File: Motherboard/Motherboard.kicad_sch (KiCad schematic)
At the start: 0 parts

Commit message: does like everything
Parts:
- added C1, C3, C4: 10uF, PCM_JLCPCB:C_0805, symbol PCM_JLCPCB-Capacitors:0805,10uF
- added C2, C5, C6, C8: 100nF, PCM_JLCPCB:C_0805, symbol PCM_JLCPCB-Capacitors:0805,100nF
- added C7: 1uF, PCM_JLCPCB:C_0805, symbol PCM_JLCPCB-Capacitors:0805,1uF
- added D1: 1N5819WS, PCM_JLCPCB:D_SOD-323, symbol PCM_JLCPCB-Diodes:Schottky,1N5819WS
- added D2: Yellow, PCM_JLCPCB:D_0805, symbol PCM_JLCPCB-Diodes:LED,0805,Yellow
- added J1: GSB316441CEU, GSB316441CEU:AMPHENOL_GSB316441CEU, symbol GSB316441CEU:GSB316441CEU
- added J2, J3, J4, J5: B3B-XH-A_LF__SN_, B3B-XH-A_LF__SN_:JST_B3B-XH-A_LF__SN_, symbol B3B-XH-A_LF__SN_:B3B-XH-A_LF__SN_
- added LS1: CMT-7525-80-SMT-TR, CMT-7525-80-SMT-TR_CUD, symbol CMT-7525-80-SMT:CMT-7525-80-SMT-TR
- added Q1: HL3400A, PCM_JLCPCB:Q_SOT-23, symbol PCM_JLCPCB-Transistors:NMOS,HL3400A
- added R1: 270Ω, PCM_JLCPCB:R_0805, symbol PCM_JLCPCB-Resistors:0805,270Ω
- added R2, R3: 10kΩ, PCM_JLCPCB:R_0805, symbol PCM_JLCPCB-Resistors:0805,10kΩ
- added R4: 100Ω, PCM_JLCPCB:R_0805, symbol PCM_JLCPCB-Resistors:0805,100Ω
- added R5: 100kΩ, PCM_JLCPCB:R_0805, symbol PCM_JLCPCB-Resistors:0805,100kΩ
- added S1, S2: Tactile Button, 160gf, PCM_JLCPCB:SW-SMD_4P-L5.1-W5.1-P3.70-LS6.5-TL-2, symbol PCM_JLCPCB-Connectors_Buttons:Tactile Button, 160gf
- added U1: ESP32-S3-WROOM-1, RF_Module:ESP32-S3-WROOM-1, symbol RF_Module:ESP32-S3-WROOM-1
- added U2: USBLC6-2P6, Package_TO_SOT_SMD:SOT-666, symbol Power_Protection:USBLC6-2P6
- added U3: AMS1117, PCM_JLCPCB:SOT-223-3_L6.5-W3.4-P2.30-LS7.0-BR, symbol PCM_JLCPCB-Power:LDO, 3.3V, 1A
- added U4: MCP73831-2-MC, Package_DFN_QFN:DFN-8-1EP_3x2mm_P0.5mm_EP1.7x1.4mm, symbol Battery_Management:MCP73831-2-MC
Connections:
- new net: Q1.1 (G), R4.1
- new net: LS1.1, Q1.3 (D)
- new net: D1.2, J1.1 (VBUS), U2.5 (VBUS)
- new net: J1.2 (D-), U2.6 (I/O1)
- new net: J1.3 (D+), U2.4 (I/O2)
- new net: C2.1, C3.1, C4.1, C5.1, LS1.2, R1.1, R2.1, R3.1, U1.2 (3V3), U3.2 (VOUT), U3.4 (VOUT)
- new net: R2.2, S1.1 (A), S1.2 (B), U1.27 (IO0)
- new net: D2.2, R1.2
- new net: U1.13 (USB_D-), U2.1 (I/O1)
- new net: U1.14 (USB_D+), U2.3 (I/O2)
- new net: R4.2, R5.1, U1.20 (IO12)
- new net: J2.1, U1.21 (IO13)
- new net: J3.1, U1.22 (IO14)
- new net: C7.1, R3.2, S2.1 (A), S2.2 (B), U1.3 (EN)
- new net: J4.1, U1.8 (IO15)
- new net: J5.1, U1.9 (IO16)
- new net: C1.1, D1.1, J2.2, J3.2, J4.2, J5.2, U3.3 (VIN), U4.1 (V_{DD}), U4.2 (V_{DD})
- new net: U4.3 (V_{BAT}), U4.4 (V_{BAT})
- new net: C6.1, S1.3 (C), S1.4 (D)
- new net: C8.1, S2.3 (C), S2.4 (D)
- new net GND: C1.2, C2.2, C3.2, C4.2, C5.2, C6.2, C7.2, C8.2, D2.1, J1.4 (GND), J1.7 (GND_DRAIN), J1.SH1 (SHIELD), J1.SH2 (SHIELD__1), J2.3, J3.3, J4.3, J5.3, Q1.2 (S), R5.2, U1.1 (GND), U1.40 (GND), U1.41 (GND), U2.2 (GND), U3.1 (GND), U4.6 (V_{SS})
- no-connect marks 0 -> 34

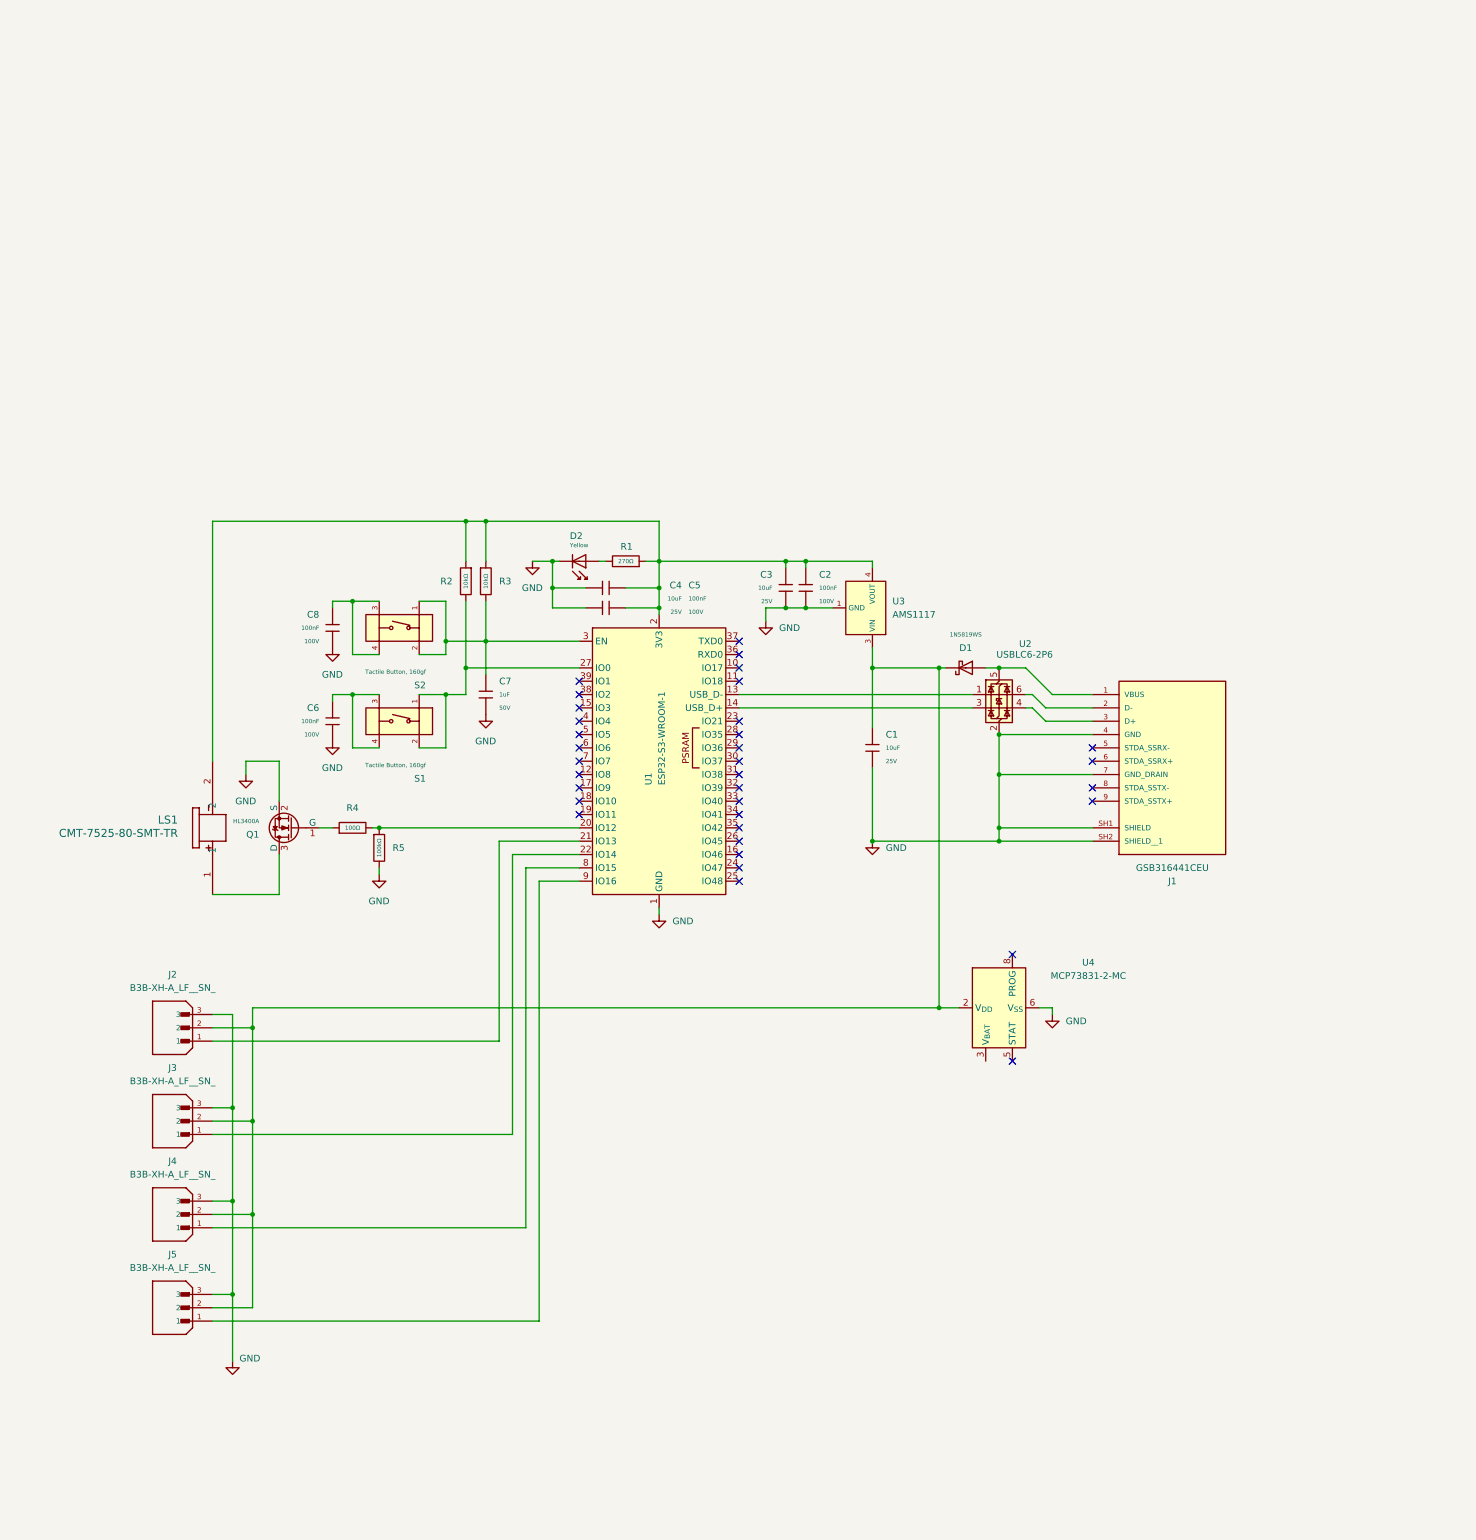
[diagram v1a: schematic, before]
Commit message: adds bms system
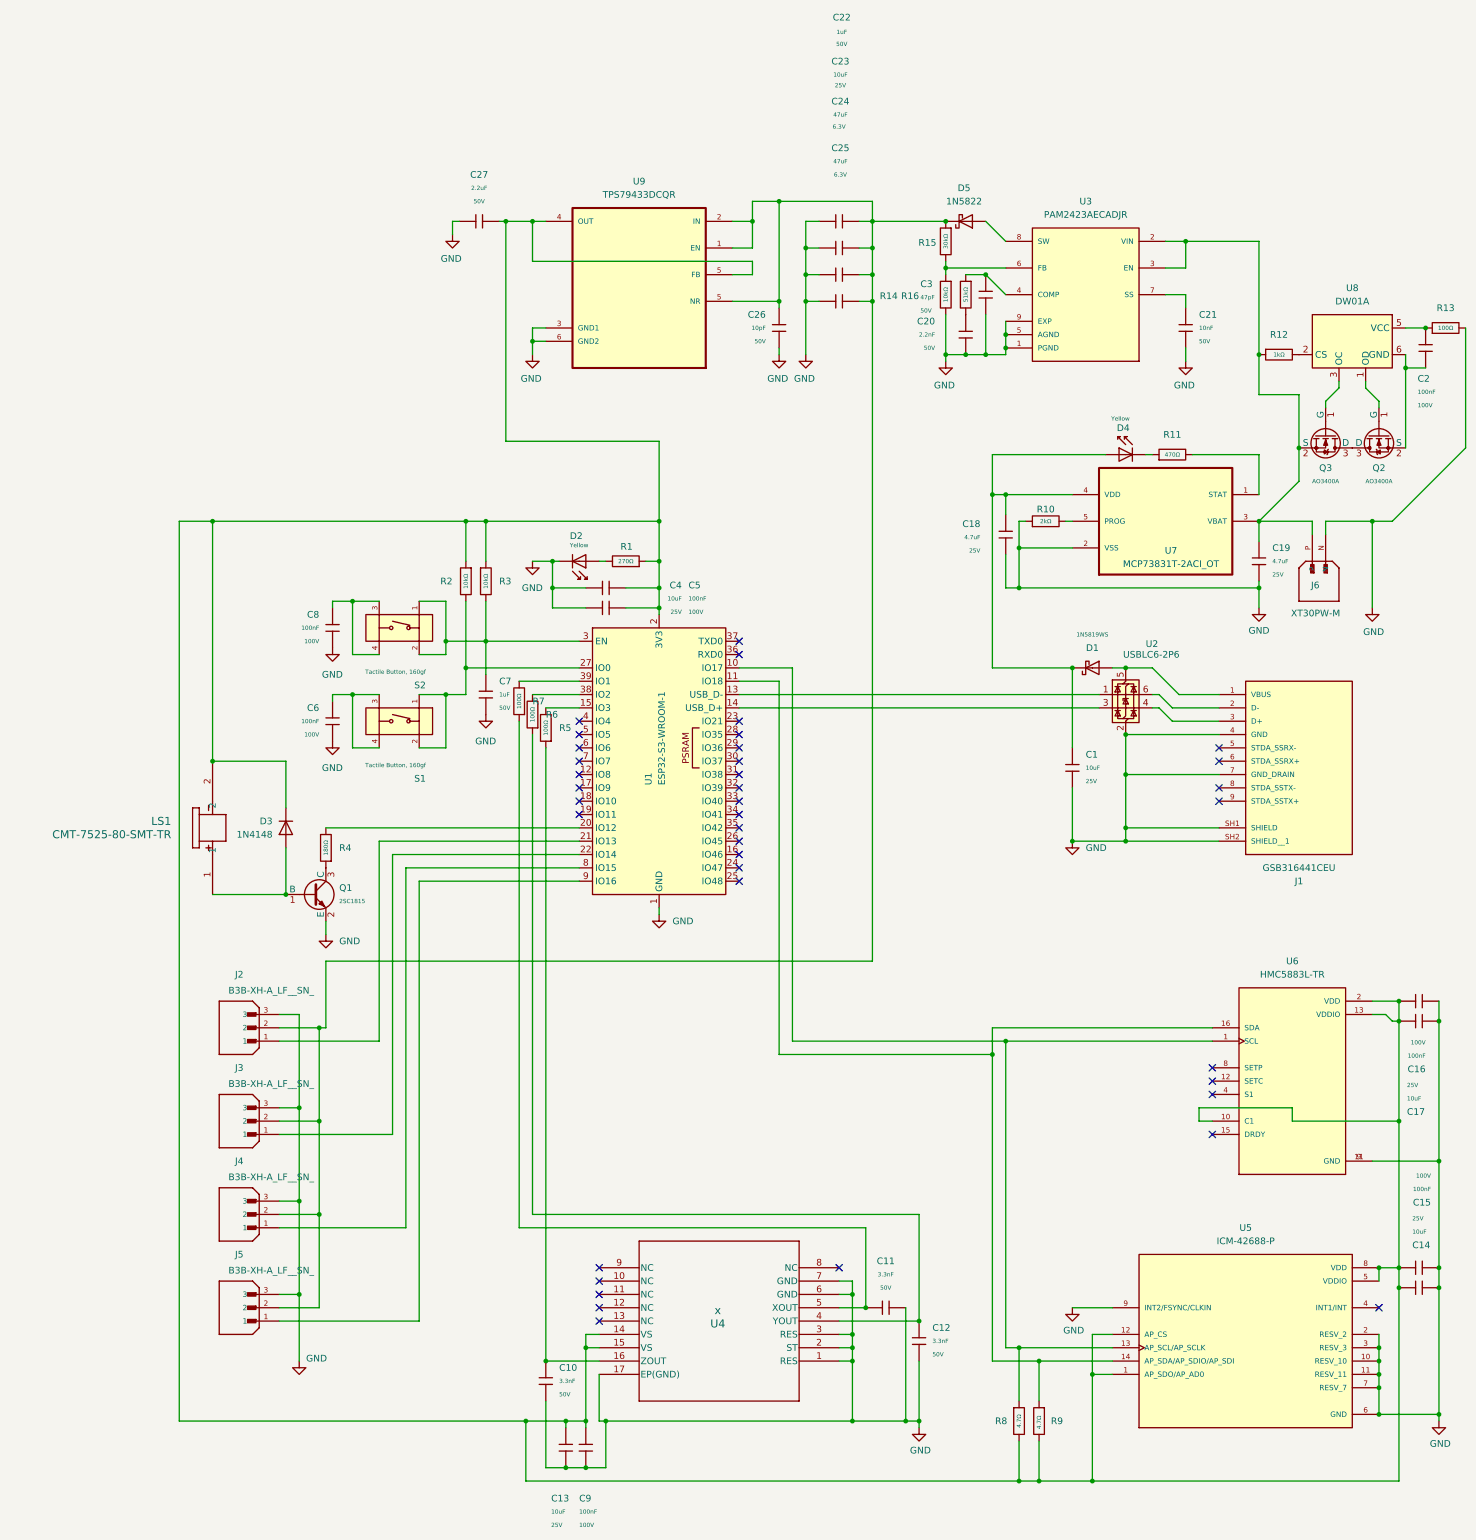
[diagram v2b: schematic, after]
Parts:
- removed C3: 10uF, PCM_JLCPCB:C_0805, symbol PCM_JLCPCB-Capacitors:0805,10uF
- removed Q1: HL3400A, PCM_JLCPCB:Q_SOT-23, symbol PCM_JLCPCB-Transistors:NMOS,HL3400A
- removed R4: 100Ω, PCM_JLCPCB:R_0805, symbol PCM_JLCPCB-Resistors:0805,100Ω
- removed R5: 100kΩ, PCM_JLCPCB:R_0805, symbol PCM_JLCPCB-Resistors:0805,100kΩ
- removed U3: AMS1117, PCM_JLCPCB:SOT-223-3_L6.5-W3.4-P2.30-LS7.0-BR, symbol PCM_JLCPCB-Power:LDO, 3.3V, 1A
- removed U4: MCP73831-2-MC, Package_DFN_QFN:DFN-8-1EP_3x2mm_P0.5mm_EP1.7x1.4mm, symbol Battery_Management:MCP73831-2-MC
- added C10, C11, C12: 3.3nF, PCM_JLCPCB:C_0603, symbol PCM_JLCPCB-Capacitors:0603,3.3nF
- added C13, C14, C17, C23: 10uF, PCM_JLCPCB:C_0805, symbol PCM_JLCPCB-Capacitors:0805,10uF
- added C15, C16, C9: 100nF, PCM_JLCPCB:C_0805, symbol PCM_JLCPCB-Capacitors:0805,100nF
- added C18, C19: 4.7uF, PCM_JLCPCB:C_0805, symbol PCM_JLCPCB-Capacitors:0805,4.7uF
- added C20: 2.2nF, PCM_JLCPCB:C_0805, symbol PCM_JLCPCB-Capacitors:0805,2.2nF
- added C21: 10nF, PCM_JLCPCB:C_0805, symbol PCM_JLCPCB-Capacitors:0805,10nF
- added C22: 1uF, PCM_JLCPCB:C_0805, symbol PCM_JLCPCB-Capacitors:0805,1uF
- added C24, C25: 47uF, PCM_JLCPCB:C_0805, symbol PCM_JLCPCB-Capacitors:0805,47uF
- added C26: 10pF, PCM_JLCPCB:C_0603, symbol PCM_JLCPCB-Capacitors:0603,10pF
- added C27: 2.2uF, PCM_JLCPCB:C_0805, symbol PCM_JLCPCB-Capacitors:0805,2.2uF
- added C3: 47pF, PCM_JLCPCB:C_0805, symbol PCM_JLCPCB-Capacitors:0805,47pF
- added D3: 1N4148, Diode_THT:D_DO-35_SOD27_P7.62mm_Horizontal, symbol Diode:1N4148
- added D4: Yellow, PCM_JLCPCB:D_0805, symbol PCM_JLCPCB-Diodes:LED,0805,Yellow
- added D5: 1N5822, Diode_THT:D_DO-201AD_P15.24mm_Horizontal, symbol Diode:1N5822
- added J6: XT30PW-M, XT30PW-M:AMASS_XT30PW-M, symbol XT30PW-M:XT30PW-M
- added Q1: 2SC1815, PCM_JLCPCB:Q_SOT-23, symbol PCM_JLCPCB-Transistors:NPN,2SC1815
- added Q2, Q3: AO3400A, PCM_JLCPCB:Q_SOT-23, symbol PCM_JLCPCB-Transistors:NMOS,AO3400A
- added R10: 2kΩ, PCM_JLCPCB:R_0805, symbol PCM_JLCPCB-Resistors:0805,2kΩ
- added R11: 470Ω, PCM_JLCPCB:R_0603, symbol PCM_JLCPCB-Resistors:0603,470Ω
- added R12: 1kΩ, PCM_JLCPCB:R_0805, symbol PCM_JLCPCB-Resistors:0805,1kΩ
- added R13: 100Ω, PCM_JLCPCB:R_0805, symbol PCM_JLCPCB-Resistors:0805,100Ω
- added R14: 10kΩ, PCM_JLCPCB:R_0805, symbol PCM_JLCPCB-Resistors:0805,10kΩ
- added R15: 30kΩ, PCM_JLCPCB:R_0805, symbol PCM_JLCPCB-Resistors:0805,30kΩ
- added R16: 51kΩ, PCM_JLCPCB:R_0805, symbol PCM_JLCPCB-Resistors:0805,51kΩ
- added R4: 180Ω, PCM_JLCPCB:R_0805, symbol PCM_JLCPCB-Resistors:0805,180Ω
- added R5, R6, R7: 100Ω, PCM_JLCPCB:R_0603, symbol PCM_JLCPCB-Resistors:0603,100Ω
- added R8, R9: 4.7Ω, PCM_JLCPCB:R_0805, symbol PCM_JLCPCB-Resistors:0805,4.7Ω
- added U3: PAM2423AECADJR, PAM2423AECADJR:SOIC127P600X163-9N, symbol PAM2423AECADJR:PAM2423AECADJR
- added U4: x, CP_16_28_ADI, symbol CP_16_28_ADI:ADXL377BCPZ-RL
- added U5: ICM-42688-P, ICM-42688-P:PQFN50P300X250X97-14N, symbol ICM-42688-P:ICM-42688-P
- added U6: HMC5883L-TR, HMC5883L-TR:XDCR_HMC5883L-TR, symbol HMC5883L-TR:HMC5883L-TR
- added U7: MCP73831T-2ACI_OT, MCP73831T-2ACI_OT:SOT95P280X145-5N, symbol MCP73831T-2ACI_OT:MCP73831T-2ACI_OT
- added U8: DW01A, Package_TO_SOT_SMD:SOT-23-6, symbol Battery_Management:DW01A
- added U9: TPS79433DCQR, TPS79433DCQR:SOT127P706X180-6N, symbol TPS79433DCQR:TPS79433DCQR
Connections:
- net GND: now also C10.1, C11.2, C12.1, C13.1, C14.1, C15.2, C16.2, C17.1, C18.1, C19.1, C20.2, C21.2, C22.1, C23.1, C24.1, C25.1, C26.2, C27.1, C3.2, C9.2, J6.N, Q1.2 (E), R10.1, R13.2, R14.2, U3.1 (PGND), U3.5 (AGND), U3.9 (EXP), U4.1 (RES), U4.17 (EP(GND)), U4.2 (ST), U4.3 (RES), U4.6 (GND), U4.7 (GND), U5.10 (RESV_10), U5.11 (RESV_11), U5.2 (RESV_2), U5.3 (RESV_3), U5.6 (GND), U5.7 (RESV_7), U5.9 (INT2/FSYNC/CLKIN), U6.11 (GND), U6.9 (GND), U7.2 (VSS), U9.3 (GND1), U9.6 (GND2); no longer C2.2
- net at LS1.1: now also D3.2 (A), Q1.1 (B)
- net at C4.1, C5.1, LS1.2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: now also C13.2, C14.2, C15.1, C16.1, C17.2, C27.2, C9.1, D3.1 (K), R8.2, R9.2, U4.14 (VS), U4.15 (VS), U5.1 (AP_SDO/AP_AD0), U5.12 (AP_CS), U5.5 (VDDIO), U5.8 (VDD), U6.10 (C1), U6.13 (VDDIO), U6.2 (VDD), U9.4 (OUT), U9.5 (NR); no longer C2.1
- net at U1.10 (IO17): now also R8.1, U5.13 (AP_SCL/AP_SCLK), U6.1 (SCL)
- net at U1.11 (IO18): now also R9.1, U5.14 (AP_SDA/AP_SDIO/AP_SDI), U6.16 (SDA)
- net at U1.15 (IO3): now also R5.2
- net at U1.20 (IO12): now also R4.2
- net at U1.38 (IO2): now also R6.2
- net at U1.39 (IO1): now also R7.2
- net at J2.2, J3.2, J4.2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: now also C22.2, C23.2, C24.2, C25.2, C26.1, D5.1 (K), R15.1, U9.1 (EN), U9.2 (IN), U9.5 (NR); no longer C1.1, D1.1
- new net: C2.1, R13.1, U8.5 (VCC)
- new net: C2.2, Q2.2 (S), U8.6 (GND)
- new net: Q2.1 (G), U8.1 (OD)
- new net: R12.2, U8.2 (CS)
- new net: Q3.1 (G), U8.3 (OC)
- new net: D5.2 (A), U3.8 (SW)
- new net: C11.1, R7.1, U4.5 (XOUT)
- new net: R10.2, U7.5 (PROG)
- new net: C19.2, J6.P, Q3.2 (S), R12.1, U3.2 (VIN), U3.3 (EN), U7.3 (VBAT)
- new net: D4.1, R11.1
- new net: C1.1, C18.2, D1.1, D4.2, U7.4 (VDD)
- new net: Q1.3 (C), R4.1
- new net: C20.1, R16.2
- new net: Q2.3 (D), Q3.3 (D)
- new net: C3.1, R16.1, U3.4 (COMP)
- new net: R14.1, R15.2, U3.6 (FB)
- new net: C21.1, U3.7 (SS)
- new net: C10.2, R5.1, U4.16 (ZOUT)
- new net: R11.2, U7.1 (STAT)
- new net: C12.2, R6.1, U4.4 (YOUT)
- no-connect marks 34 -> 38
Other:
- moved on the sheet: C1, D1, J1, J2, J3, J4, J5, U2

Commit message: added bms system + buck converter
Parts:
- removed C18, C19: 4.7uF, PCM_JLCPCB:C_0805, symbol PCM_JLCPCB-Capacitors:0805,4.7uF
- removed C20: 2.2nF, PCM_JLCPCB:C_0805, symbol PCM_JLCPCB-Capacitors:0805,2.2nF
- removed C21: 10nF, PCM_JLCPCB:C_0805, symbol PCM_JLCPCB-Capacitors:0805,10nF
- removed C22: 1uF, PCM_JLCPCB:C_0805, symbol PCM_JLCPCB-Capacitors:0805,1uF
- removed C23: 10uF, PCM_JLCPCB:C_0805, symbol PCM_JLCPCB-Capacitors:0805,10uF
- removed C24, C25: 47uF, PCM_JLCPCB:C_0805, symbol PCM_JLCPCB-Capacitors:0805,47uF
- removed C3: 47pF, PCM_JLCPCB:C_0805, symbol PCM_JLCPCB-Capacitors:0805,47pF
- removed C6: 100nF, PCM_JLCPCB:C_0805, symbol PCM_JLCPCB-Capacitors:0805,100nF
- removed D1: 1N5819WS, PCM_JLCPCB:D_SOD-323, symbol PCM_JLCPCB-Diodes:Schottky,1N5819WS
- removed D5: 1N5822, Diode_THT:D_DO-201AD_P15.24mm_Horizontal, symbol Diode:1N5822
- removed J1: GSB316441CEU, GSB316441CEU:AMPHENOL_GSB316441CEU, symbol GSB316441CEU:GSB316441CEU
- removed J6: XT30PW-M, XT30PW-M:AMASS_XT30PW-M, symbol XT30PW-M:XT30PW-M
- removed Q2, Q3: AO3400A, PCM_JLCPCB:Q_SOT-23, symbol PCM_JLCPCB-Transistors:NMOS,AO3400A
- removed R10: 2kΩ, PCM_JLCPCB:R_0805, symbol PCM_JLCPCB-Resistors:0805,2kΩ
- removed R11: 470Ω, PCM_JLCPCB:R_0603, symbol PCM_JLCPCB-Resistors:0603,470Ω
- removed R12: 1kΩ, PCM_JLCPCB:R_0805, symbol PCM_JLCPCB-Resistors:0805,1kΩ
- removed R13: 100Ω, PCM_JLCPCB:R_0805, symbol PCM_JLCPCB-Resistors:0805,100Ω
- removed R14: 10kΩ, PCM_JLCPCB:R_0805, symbol PCM_JLCPCB-Resistors:0805,10kΩ
- removed R16: 51kΩ, PCM_JLCPCB:R_0805, symbol PCM_JLCPCB-Resistors:0805,51kΩ
- removed U3: PAM2423AECADJR, PAM2423AECADJR:SOIC127P600X163-9N, symbol PAM2423AECADJR:PAM2423AECADJR
- removed U7: MCP73831T-2ACI_OT, MCP73831T-2ACI_OT:SOT95P280X145-5N, symbol MCP73831T-2ACI_OT:MCP73831T-2ACI_OT
- removed U8: DW01A, Package_TO_SOT_SMD:SOT-23-6, symbol Battery_Management:DW01A
- added C18, C20, C21, C6: 1uF, PCM_JLCPCB:C_0805, symbol PCM_JLCPCB-Capacitors:0805,1uF
- added C19, C24, C29: 100nF, PCM_JLCPCB:C_0805, symbol PCM_JLCPCB-Capacitors:0805,100nF
- added C22, C30: 22uF, PCM_JLCPCB:C_0805, symbol PCM_JLCPCB-Capacitors:0805,22uF
- added C23: CSEG1060-3R3M, CAP_CSEG1060-3R3M_COD, symbol CSEG1060-3R3M:CSEG1060-3R3M
- added C25: 15pF, PCM_JLCPCB:C_0805, symbol PCM_JLCPCB-Capacitors:0805,15pF
- added C28: 22nF, PCM_JLCPCB:C_0805, symbol PCM_JLCPCB-Capacitors:0805,22nF
- added C3: 2.2uF, PCM_JLCPCB:C_0805, symbol PCM_JLCPCB-Capacitors:0805,2.2uF
- added D1: Yellow, PCM_JLCPCB:D_0805, symbol PCM_JLCPCB-Diodes:LED,0805,Yellow
- added J1: USB4056-03-A_REVA2, Custom Components:GCT_USB4056-03-A_REVA2, symbol USB4056-03-A_REVA2:USB4056-03-A_REVA2
- added J6: B3B-XH-A_LF__SN_, B3B-XH-A_LF__SN_:JST_B3B-XH-A_LF__SN_, symbol B3B-XH-A_LF__SN_:B3B-XH-A_LF__SN_
- added J7: XT30PW-M, XT30PW-M:AMASS_XT30PW-M, symbol XT30PW-M:XT30PW-M
- added L1: B82462G4152M000, B82462G4152M000:IND_B82462G4152M000, symbol B82462G4152M000:B82462G4152M000
- added MOSFET1, MOSFET2: SI4838BDY-T1-GE3, SOIC8_NARROW_VIS, symbol SI4838BDY-T1-GE3:SI4838BDY-T1-GE3
- added Q2: MDD2301, PCM_JLCPCB:Q_SOT-23, symbol PCM_JLCPCB-Transistors:PMOS,MDD2301
- added R10: 180Ω, PCM_JLCPCB:R_0805, symbol PCM_JLCPCB-Resistors:0805,180Ω
- added R11, R12: 150Ω, PCM_JLCPCB:R_0805, symbol PCM_JLCPCB-Resistors:0805,150Ω
- added R13: 3.9kΩ, PCM_JLCPCB:R_0805, symbol PCM_JLCPCB-Resistors:0805,3.9kΩ
- added R14, R20: 270Ω, PCM_JLCPCB:R_0805, symbol PCM_JLCPCB-Resistors:0805,270Ω
- added R16, R17, R21, R28: 5.1kΩ, PCM_JLCPCB:R_0805, symbol PCM_JLCPCB-Resistors:0805,5.1kΩ
- added R18: 10kΩ, PCM_JLCPCB:R_0603, symbol PCM_JLCPCB-Resistors:0603,10kΩ
- added R19: 6.2kΩ, PCM_JLCPCB:R_0805, symbol PCM_JLCPCB-Resistors:0805,6.2kΩ
- added R22: 22kΩ, PCM_JLCPCB:R_0805, symbol PCM_JLCPCB-Resistors:0805,22kΩ
- added R23: 100kΩ, PCM_JLCPCB:R_0805, symbol PCM_JLCPCB-Resistors:0805,100kΩ
- added R24: 39kΩ, PCM_JLCPCB:R_0805, symbol PCM_JLCPCB-Resistors:0805,39kΩ
- added R25: 33kΩ, PCM_JLCPCB:R_0805, symbol PCM_JLCPCB-Resistors:0805,33kΩ
- added R26: 10kΩ, PCM_JLCPCB:R_0805, symbol PCM_JLCPCB-Resistors:0805,10kΩ
- added R27: 47kΩ, PCM_JLCPCB:R_0805, symbol PCM_JLCPCB-Resistors:0805,47kΩ
- added RT1: NCU15XH103F6SRC, NCU15XH103F6SRC:THRMC1005X55N, symbol NCU15XH103F6SRC:NCU15XH103F6SRC
- added U3: TPS56A37RPAR, RPA0010A-MFG, symbol TPS56A37RPAR:TPS56A37RPAR
- added U7: MP2672AGD-0000-P, QFN-18_MP2672A_MNP, symbol MP2672A:MP2672AGD-0000-P
- added U8: S-8252ABE-M6T1U, SOT236-A-PKG_MP006-A-P-SD-2.1_ABL, symbol S-8252ABE-M6T1U:S-8252ABE-M6T1U
- J2, J3, J4, J5: footprint B3B-XH-A_LF__SN_:JST_B3B-XH-A_LF__SN_ -> Custom Components:JST_B3B-XH-A_LF__SN_
- U4: value x -> ADXL377; footprint CP_16_28_ADI -> Custom Components:CP_16_28_ADI
- U5: footprint ICM-42688-P:PQFN50P300X250X97-14N -> Custom Components:PQFN50P300X250X97-14N
- U6: footprint HMC5883L-TR:XDCR_HMC5883L-TR -> Custom Components:XDCR_HMC5883L-TR
- U9: footprint TPS79433DCQR:SOT127P706X180-6N -> Custom Components:SOT127P706X180-6N
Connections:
- net GND: now also C2.2, S1.3 (C), S1.4 (D), S2.3 (C), S2.4 (D), C20.2, C21.2, C22.1, C28.2, C29.2, C3.1, C30.2, J1.A1 (GND_A), J1.A12 (GND_A), J1.B1 (GND_B), J1.B12 (GND_B), J1.S1 (SHELL_GND), J1.S2 (SHELL_GND), J1.S3 (SHELL_GND), J1.S4 (SHELL_GND), MOSFET1.1, MOSFET1.2, MOSFET1.3, R10.2, R16.2, R17.1, R18.2, R19.1, R27.2, R28.2, RT1.1, U7.13 (PGND), U7.6 (AGND)
- net at C13.2, C27.2, C4.1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: no longer C14.2, C15.1, C16.1, C17.2, R8.2, R9.2, U5.1 (AP_SDO/AP_AD0), U5.12 (AP_CS), U5.5 (VDDIO), U5.8 (VDD), U6.10 (C1), U6.13 (VDDIO), U6.2 (VDD), U9.5 (NR)
- net at C2.1: now also R2.2, S1.1 (A), S1.2 (B), U1.27 (IO0)
- net at J2.2, J3.2, J4.2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: now also C1.1, C3.2, L1.1, Q2.2 (S), R14.2, R23.1, U7.1 (IN); no longer C26.1, U9.5 (NR)
- net at U2.5 (VBUS): now also J1.A4 (VBUS_A), J1.A9 (VBUS_A), J1.B4 (VBUS_B), J1.B9 (VBUS_B), Q2.3 (D)
- net at U2.6 (I/O1): now also J1.A7 (DN1), J1.B6 (DP2)
- net at U2.4 (I/O2): now also J1.A6 (DP1), J1.B7 (DN2)
- net at C7.1, R3.2, S2.1 (A)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: now also C8.1
- net at D4.1: now also U7.16 (*STAT)
- net at D4.2: now also R20.2; no longer C1.1
- net at D3.2 (A), LS1.1: now also Q1.3 (C); no longer Q1.1 (B)
- net at R4.1: now also Q1.1 (B); no longer Q1.3 (C)
- net at R15.2: now also R18.1, U7.7 (VLIM)
- new net: C14.2, C15.1, C16.1, C17.2, R8.2, R9.2, U5.1 (AP_SDO/AP_AD0), U5.12 (AP_CS), U5.5 (VDDIO), U5.8 (VDD), U6.10 (C1), U6.13 (VDDIO), U6.2 (VDD)
- new net: C20.1, R20.1, R21.1, U7.4 (VCC)
- new net: C26.1, U9.5 (NR)
- new net: C23.1, C25.1, R24.1, R25.1
- new net: C25.2, R24.2, R25.2, R26.1, U3.2 (FB)
- new net: R27.1, R28.1, U3.10 (MODE)
- new net: R22.2, RT1.2
- new net: R13.1, U8.3 (VM)
- new net: C18.2, C6.1, J6.3, J7.N, MOSFET2.1, MOSFET2.2, MOSFET2.3, R13.2, U8.6 (VSS)
- new net: C22.2, C29.1, C30.1, J6.1, J7.P, R11.2, U3.8 (VIN), U7.10 (BATT)
- new net: J6.2, R12.2, U7.9 (MID)
- new net: C21.1, U7.11 (SYS)
- new net: C6.2, R11.1, U8.5 (VDD)
- new net: R21.2, R22.1, U7.8 (NTC)
- new net: J1.A5 (CC1), R17.2
- new net: J1.B5 (CC2), R16.1
- new net: C28.1, U3.5 (SS)
- new net: Q2.1 (G), R10.1
- new net: C23.2, C24.1, U3.6 (SW)
- new net: D1.2, R14.1
- new net: MOSFET2.4, U8.2 (CO)
- new net: MOSFET1.5, MOSFET1.6, MOSFET1.7, MOSFET1.8, MOSFET2.5, MOSFET2.6, MOSFET2.7, MOSFET2.8
- new net: R26.2, U3.3 (AGND), U3.9 (PGND)
- new net: C24.2, U3.7 (BOOT)
- new net: MOSFET1.4, U8.1 (DO)
- new net: C18.1, R12.1, U8.4 (VC)
- new net: C19.2, L1.2, U7.12 (SW), U7.2 (SW)
- new net: R23.2, U3.4 (PG)
- new net: R19.2, U7.5 (ISET)
- new net: D1.1, U7.18 (*ACOK)
- new net: C19.1, U7.3 (BST)
- no-connect marks 38 -> 48
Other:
- moved on the sheet: C1, C10, C11, C12, C13, C14, C15, C16, C17, C26, C27, C4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
